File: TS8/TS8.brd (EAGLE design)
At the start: 13 x 11.6 mm, 4 parts, among them J1 CONN_3, J2 CONN_3

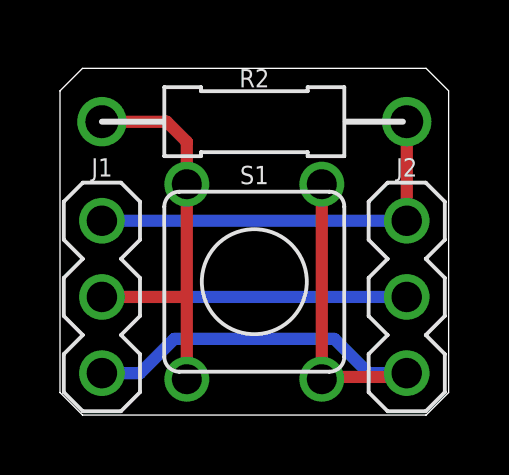
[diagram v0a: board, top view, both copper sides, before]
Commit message: Backlog of various boards
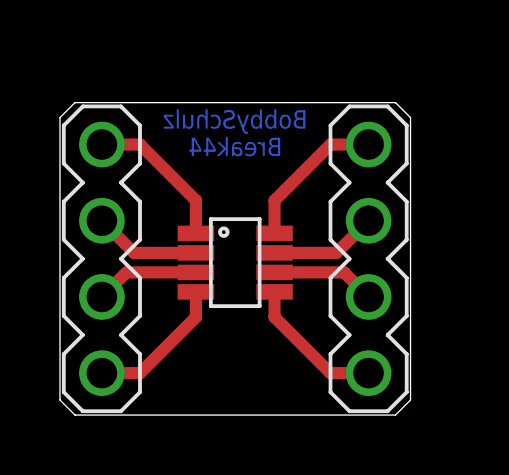
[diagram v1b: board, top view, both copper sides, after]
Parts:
- removed J1: CONN_3, bschulz:1X03
- removed R2: 10k, bschulz_passives:R_TH_0.4"
- removed S1: BUTTON6X6_TH, bschulz:SWITCH_6MM_TH
- added J3: CONN_42.54, bschulz:1X04
- added U1: GEN_8TS8, bschulz:TS8
- J2: value CONN_3 -> CONN_42.54; device bschulz:1X03 -> bschulz:1X04
- moved J2 1.80 mm to (10.3, 5.21)
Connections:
- removed net P1: J1.3, J2.3, S1.3, S1.4
- removed net P2: J1.2, J2.2, R2.P$1, S1.1, S1.2
- removed net P3: J1.1, J2.1, R2.P$2
- new net 1: J3.1, U1.1
- new net 2: J3.2, U1.2
- new net 3: J3.3, U1.3
- new net 4: J3.4, U1.4
- new net 5: J2.4, U1.5
- new net 6: J2.3, U1.6
- new net 7: J2.2, U1.7
- new net 8: J2.1, U1.8
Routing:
- net P2: track 24.0 -> 0.00 mm
- net P1: track 20.5 -> 0.00 mm
- net P3: track 13.5 -> 0.00 mm
- net 8: track 0.00 -> 5.00 mm
- net 1: track 0.00 -> 5.00 mm
- net 5: track 0.00 -> 4.75 mm
- net 4: track 0.00 -> 4.75 mm
- net 7: track 0.00 -> 3.58 mm
- net 2: track 0.00 -> 3.58 mm
- net 6: track 0.00 -> 3.47 mm
- net 3: track 0.00 -> 3.47 mm
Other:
- board size 13 x 11.6 mm -> 11.7 x 10.4 mm
- board text added: "4"
- board text added: "5"
- board text added: "6"
- board text added: "7"
- board text added: "8"
- board text added: "BobbySchulz Break44"
- board text added: "TS8"
- board text removed: "B. Schulz Break44"
- board text removed: "v1.0"
